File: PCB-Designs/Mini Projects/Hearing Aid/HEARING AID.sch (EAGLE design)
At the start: 22 parts, among them T1 BC547, T2 BC547, T3 BC547, T4 BC547

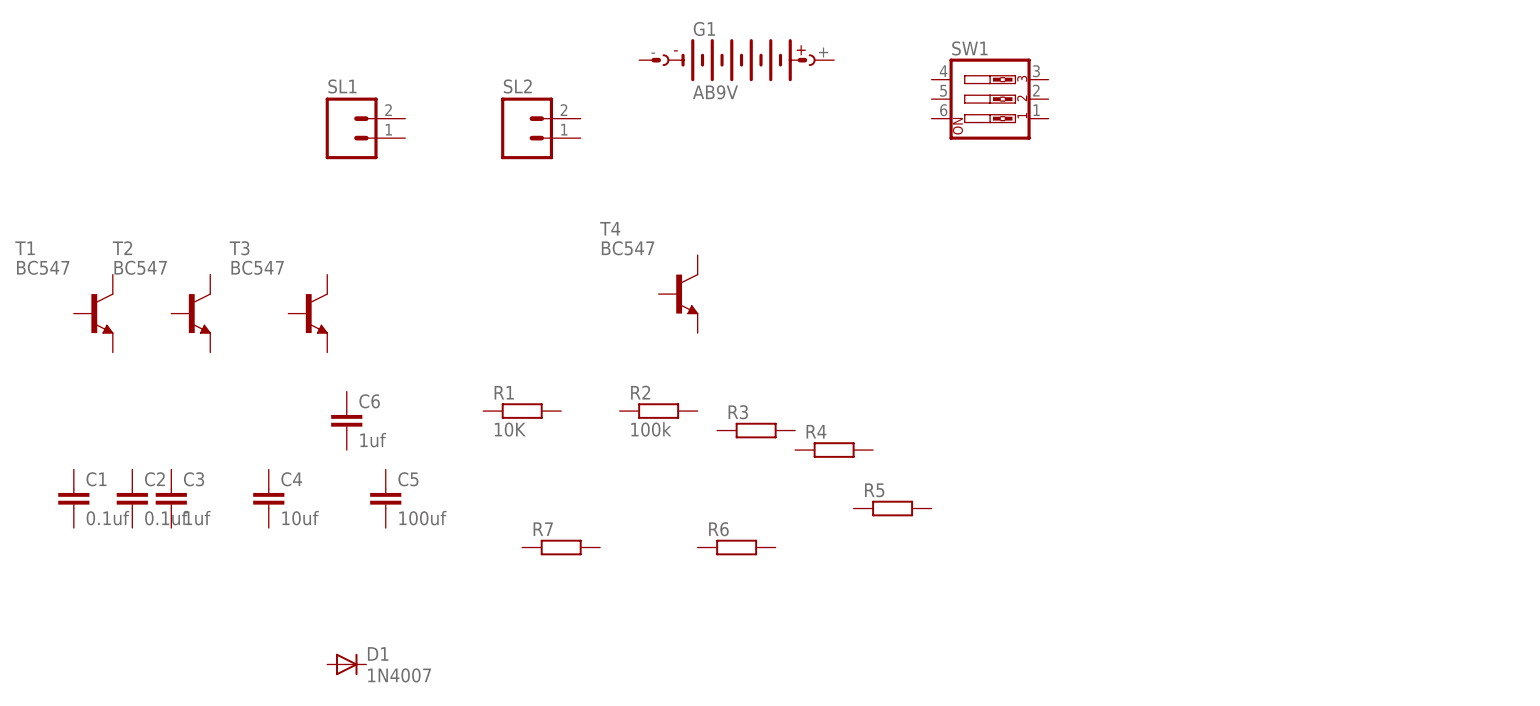
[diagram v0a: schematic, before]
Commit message: add
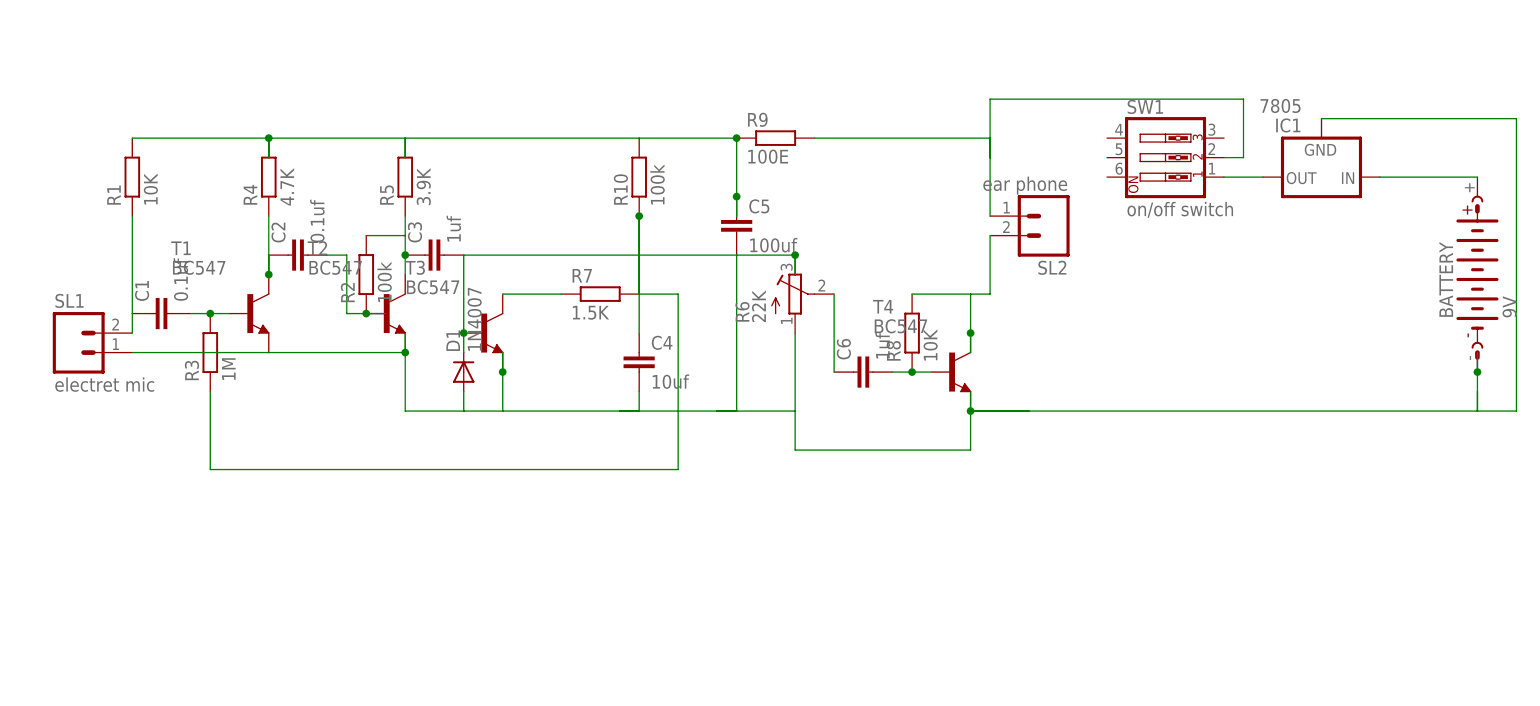
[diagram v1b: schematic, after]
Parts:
- removed G1: AB9V, battery:AB9V
- added BATTERY: 9V, battery:AB9V
- added IC1: 7805, v-reg:78XXL
- added R10: 100k, rcl:R-EU_0204/7
- added R8: 10K, rcl:R-EU_0204/7
- added R9: 100E, rcl:R-EU_0204/7
- R3: value (none) -> 1M
- R4: value (none) -> 4.7K
- R5: value (none) -> 3.9K
- R6: value (none) -> 22K; device rcl:R-EU_0204/7 -> resistor:R-TRIMM64P
- R7: value (none) -> 1.5K
- SL1: value (none) -> electret mic
- SL2: value (none) -> ear phone
- SW1: value (none) -> on/off switch
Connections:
- new net N$1: C1.2, R3.2, T1.B
- new net N$10: C5.1, R1.2, R10.2, R4.2, R5.2, R9.1
- new net N$12: C6.1, R6.S
- new net N$13: C6.2, R8.1, T4.B
- new net N$14: R8.2, SL2.2, T4.C
- new net N$16: BATTERY.+, IC1.IN
- new net N$17: BATTERY.-, C4.2, C5.2, D1.A, IC1.GND, R6.E, SL1.1, T1.E, T2.E, T3.E, T4.E
- new net N$18: IC1.OUT, SW1.1
- new net N$19: R9.2, SL2.1, SW1.2
- new net N$2: C1.1, R1.1, SL1.2
- new net N$3: C2.1, R4.1, T1.C
- new net N$4: C2.2, R2.1, T2.B
- new net N$5: C3.1, R2.2, R5.1, T2.C
- new net N$6: C3.2, D1.C, R6.A, T3.B
- new net N$7: R7.1, T3.C
- new net N$8: C4.1, R10.1, R3.1, R7.2
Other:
- moved on the sheet: C1, C2, C3, C4, C5, C6, D1, R1, R2, R3, R4, R5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
